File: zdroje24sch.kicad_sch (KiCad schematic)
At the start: 8 parts, among them J2 Conn_02x05_Top_Bottom

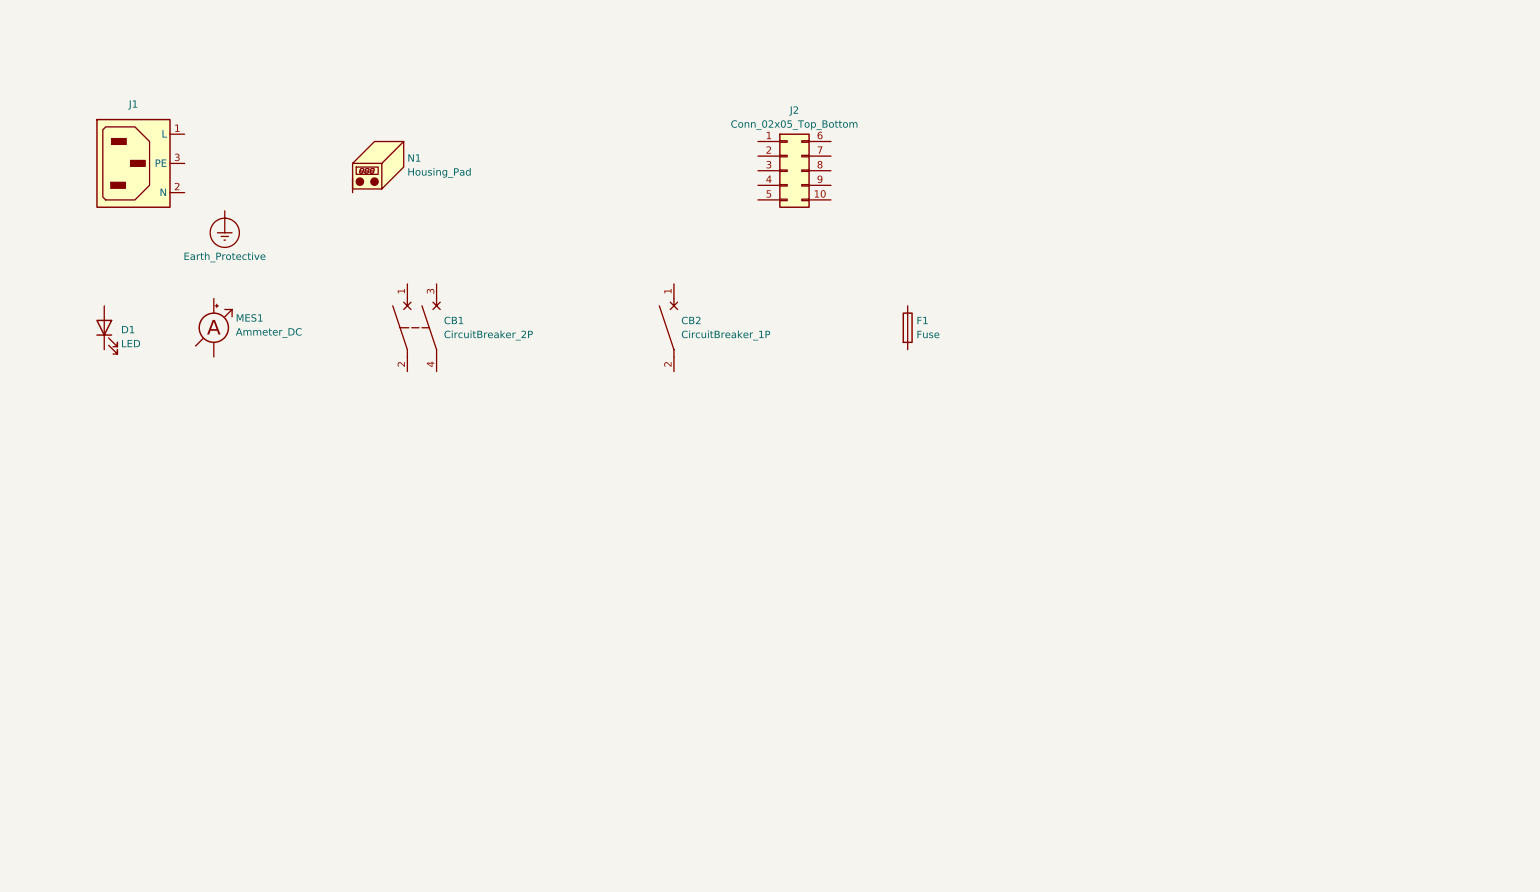
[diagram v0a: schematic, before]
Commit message: Zapojit vse.
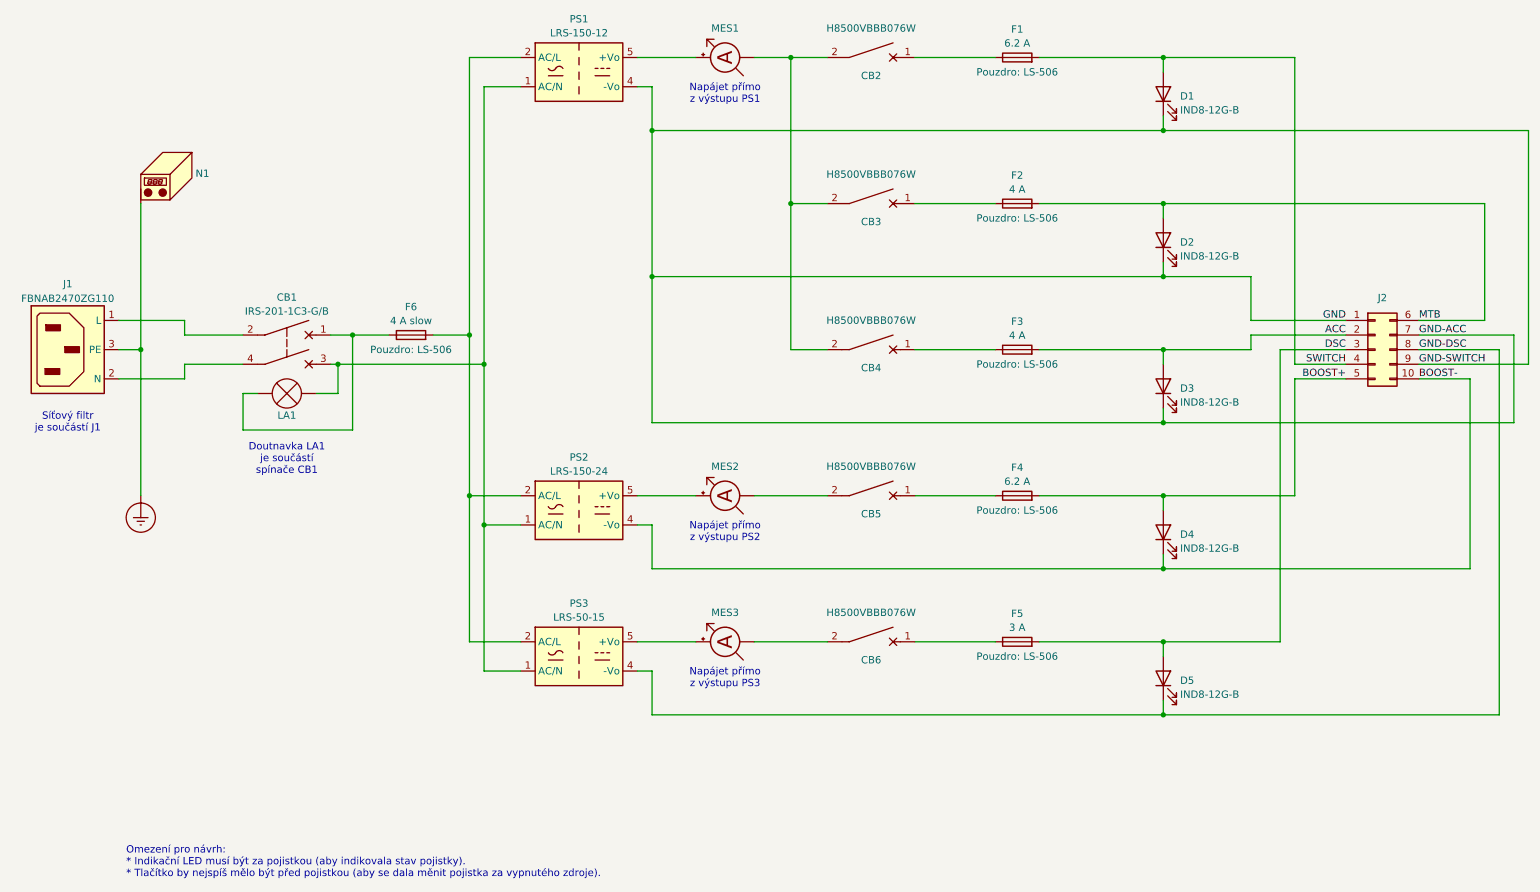
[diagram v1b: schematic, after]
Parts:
- added CB3, CB4, CB5, CB6: H8500VBBB076W, symbol Device:CircuitBreaker_1P
- added D2, D3, D4, D5: IND8-12G-B, symbol Device:LED
- added F2, F3: 4 A, symbol Device:Fuse
- added F4: 6.2 A, symbol Device:Fuse
- added F5: 3 A, symbol Device:Fuse
- added F6: 4 A slow, symbol Device:Fuse
- added LA1: ~, symbol Device:Lamp
- added MES2, MES3: ~, symbol Device:Ammeter_DC
- added PS1: LRS-150-12, Converter_ACDC:Converter_ACDC_Murata_BAC05SxxDC_THT, symbol Converter_ACDC:BAC05S05DC
- added PS2: LRS-150-24, Converter_ACDC:Converter_ACDC_Murata_BAC05SxxDC_THT, symbol Converter_ACDC:BAC05S05DC
- added PS3: LRS-50-15, Converter_ACDC:Converter_ACDC_Murata_BAC05SxxDC_THT, symbol Converter_ACDC:BAC05S05DC
- CB1: value CircuitBreaker_2P -> IRS-201-1C3-G/B
- CB2: value CircuitBreaker_1P -> H8500VBBB076W
- D1: value LED -> IND8-12G-B
- F1: value Fuse -> 6.2 A; Pouzdro (none) -> LS-506
- J1: value ~ -> FBNAB2470ZG110
- J2: value Conn_02x05_Top_Bottom -> ~
- MES1: value Ammeter_DC -> ~
- N1: value Housing_Pad -> ~
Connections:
- net at N1.1 (PAD): now also J1.3 (PE)
- net GND: now reaches J2.1 (Pin_1)
- net GND: now also D1.1 (K), J2.7 (Pin_7), J2.9 (Pin_9), D2.1 (K), D3.1 (K), PS1.4 (-Vo)
- net BOOST-: now reaches J2.10 (Pin_10)
- net BOOST-: now also D4.1 (K), PS2.4 (-Vo)
- net ACC: now reaches J2.2 (Pin_2)
- net ACC: now also D3.2 (A), F3.2
- net DSC: now reaches J2.3 (Pin_3)
- net DSC: now also D5.2 (A), F5.2
- net SWITCH: now reaches J2.4 (Pin_4)
- net SWITCH: now also D1.2 (A), F1.2
- net BOOST+: now reaches J2.5 (Pin_5)
- net BOOST+: now also D4.2 (A), F4.2
- net MTB: now reaches J2.6 (Pin_6)
- net MTB: now also D2.2 (A), F2.2
- net GND-DSC: now reaches J2.8 (Pin_8)
- net GND-DSC: now also D5.1 (K), PS3.4 (-Vo)
- net at CB2.1: now also F1.1
- net at CB2.2: now also MES1.1 (-), CB3.2, CB4.2
- net at CB1.1: now also F6.1, LA1.1 (-)
- net at CB1.2: now also J1.1 (L)
- net at CB1.3: now also LA1.2 (+), PS1.1 (AC/N), PS2.1 (AC/N), PS3.1 (AC/N)
- net at CB1.4: now also J1.2 (N)
- net at MES1.2 (+): now also PS1.5 (+Vo)
- new net: CB5.1, F4.1
- new net: CB6.1, F5.1
- new net: CB6.2, MES3.1 (-)
- new net: CB3.1, F2.1
- new net: F6.2, PS1.2 (AC/L), PS2.2 (AC/L), PS3.2 (AC/L)
- new net: CB4.1, F3.1
- new net: MES2.2 (+), PS2.5 (+Vo)
- new net: CB5.2, MES2.1 (-)
- new net: MES3.2 (+), PS3.5 (+Vo)
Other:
- note added: "Doutnavka LA1 je součástí spínače CB1"
- note added: "Napájet přímo z výstupu PS1"
- note added: "Napájet přímo z výstupu PS2"
- note added: "Napájet přímo z výstupu PS3"
- note added: "Omezení pro návrh: * Indikační LED musí být za pojistkou (aby indikovala stav pojistky). * Tlačítko by nejspíš mělo být před pojistkou (aby se dala měnit pojistka za vypnutého zdroje)."
- note added: "Síťový filtr je součástí J1"
- title: (none) -> Napájecí zdroj KMŽ/LRKV 2024/2025
- moved on the sheet: CB1, CB2, D1, F1, J1, J2, MES1, N1
